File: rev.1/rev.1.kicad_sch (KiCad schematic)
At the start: 129 parts, among them Q1 BC857, Q2 BC817, SW1 RESET, SW2 POWER, X1 POWER, X2 Манипулятор_1, X3 AUDIO_1, X4 AUDIO_2, X5 Манипулятор_2, X6 VIDEO

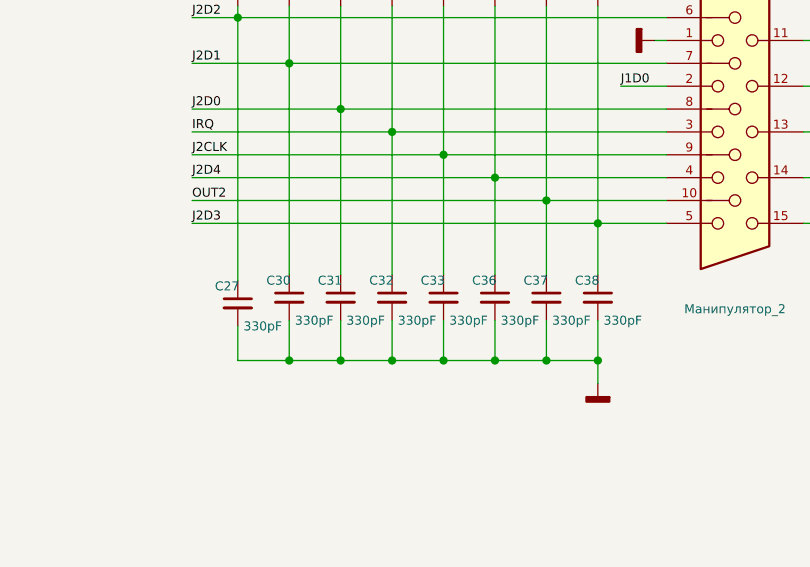
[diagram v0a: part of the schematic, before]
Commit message: раставил элементы приступил к трассеровке
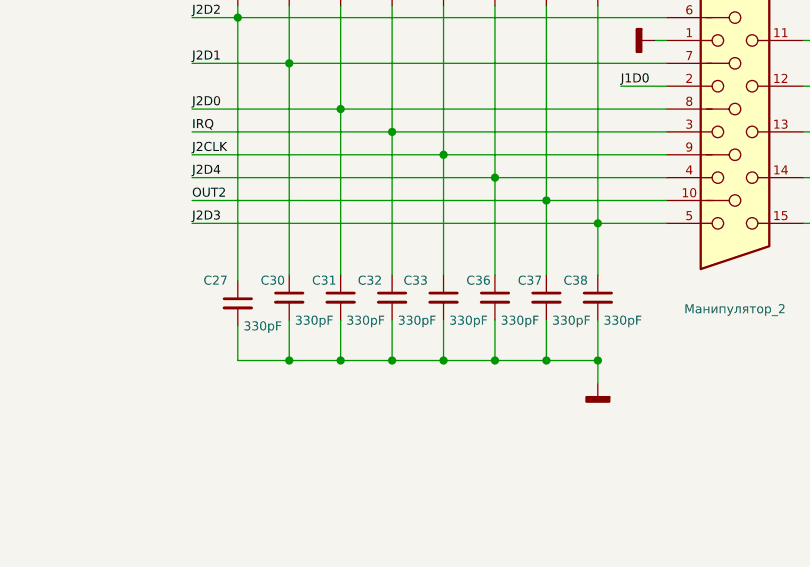
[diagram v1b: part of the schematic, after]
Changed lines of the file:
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@@
   (symbol (lib_id "Device:C_Small") (at 513.08 71.755 0) (unit 1)
     (in_bom yes) (on_board yes) (dnp no)
-    (property "Reference" "C33" (at 510.54 69.85 0)
+    (property "Reference" "C33" (at 508.635 69.85 0)
       (effects (font (size 1 1)) (justify left))
     )
@@
   (symbol (lib_id "Device:C_Small") (at 518.795 71.755 0) (unit 1)
     (in_bom yes) (on_board yes) (dnp no)
-    (property "Reference" "C36" (at 516.255 69.85 0)
+    (property "Reference" "C36" (at 515.62 69.85 0)
       (effects (font (size 1 1)) (justify left))
     )
@@
   (symbol (lib_id "Device:C_Small") (at 501.65 71.755 0) (unit 1)
     (in_bom yes) (on_board yes) (dnp no)
-    (property "Reference" "C31" (at 499.11 69.85 0)
+    (property "Reference" "C31" (at 498.475 69.85 0)
       (effects (font (size 1 1)) (justify left))
     )
@@
   (symbol (lib_id "Device:C_Small") (at 507.365 71.755 0) (unit 1)
     (in_bom yes) (on_board yes) (dnp no)
-    (property "Reference" "C32" (at 504.825 69.85 0)
+    (property "Reference" "C32" (at 503.555 69.85 0)
       (effects (font (size 1 1)) (justify left))
     )
@@
   (symbol (lib_id "Device:C_Small") (at 530.225 71.755 0) (unit 1)
     (in_bom yes) (on_board yes) (dnp no)
-    (property "Reference" "C38" (at 527.685 69.85 0)
+    (property "Reference" "C38" (at 526.415 69.85 0)
       (effects (font (size 1 1)) (justify left))
     )
@@
   (symbol (lib_id "Device:C_Small") (at 490.22 72.39 0) (unit 1)
     (in_bom yes) (on_board yes) (dnp no)
-    (property "Reference" "C27" (at 487.68 70.485 0)
+    (property "Reference" "C27" (at 486.41 69.85 0)
       (effects (font (size 1 1)) (justify left))
     )
@@
   (symbol (lib_id "Device:C_Small") (at 495.935 71.755 0) (unit 1)
     (in_bom yes) (on_board yes) (dnp no)
-    (property "Reference" "C30" (at 493.395 69.85 0)
+    (property "Reference" "C30" (at 492.76 69.85 0)
       (effects (font (size 1 1)) (justify left))
     )
@@
   (symbol (lib_id "Device:C_Small") (at 524.51 71.755 0) (unit 1)
     (in_bom yes) (on_board yes) (dnp no)
-    (property "Reference" "C37" (at 521.97 69.85 0)
+    (property "Reference" "C37" (at 521.335 69.85 0)
       (effects (font (size 1 1)) (justify left))
     )
